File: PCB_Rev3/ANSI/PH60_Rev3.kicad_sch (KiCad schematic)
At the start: 50 parts, among them J1 USB_C_Receptacle_USB2.0_16P, J2 Conn_01x02, J3 Conn_01x02_Pin, J4 Conn_01x02_Pin, J6 Conn_01x02_Pin, J8 Conn_01x02_Pin, SW1 SW_SPDT_321, U1 TLV62569DBV, U2 RP2040, U4 ETA6093, U6 W25Q16JVSS, Y1 Crystal_GND24

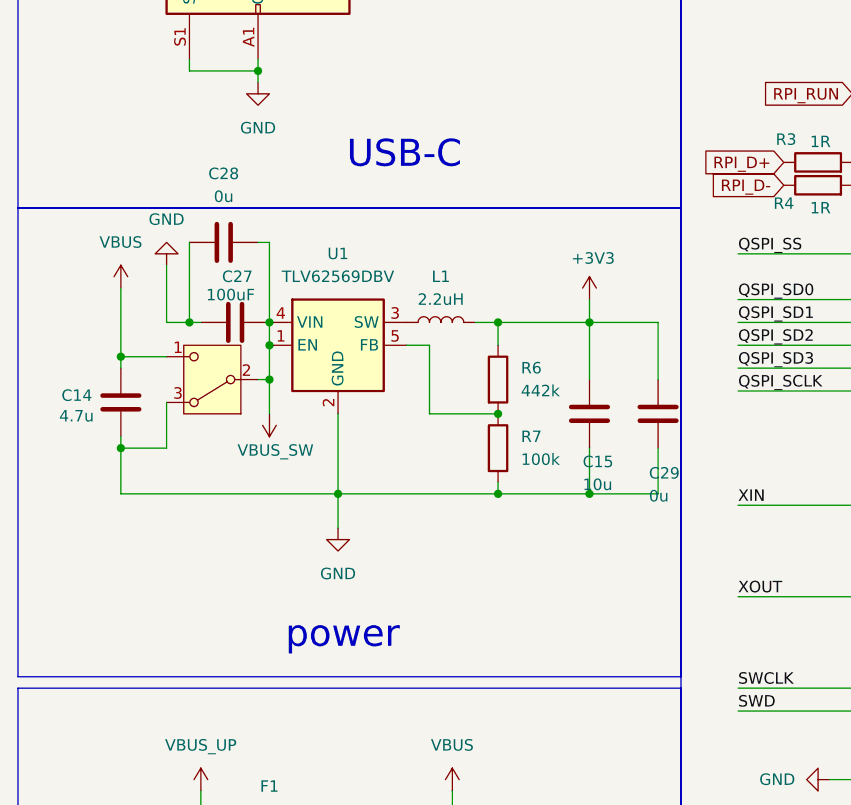
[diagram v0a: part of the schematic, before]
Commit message: Routing update
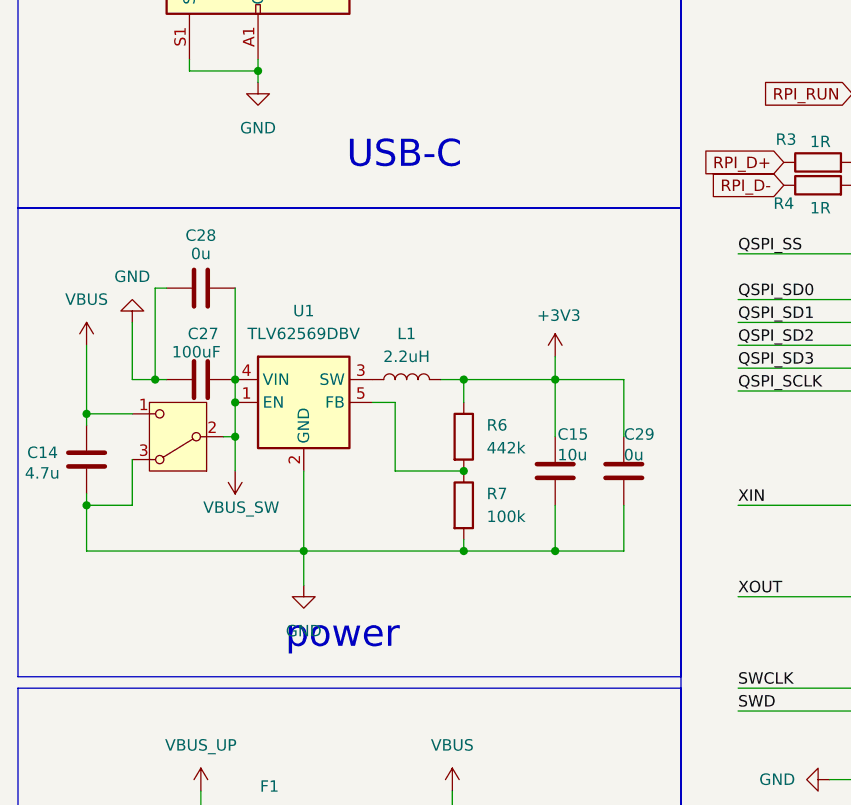
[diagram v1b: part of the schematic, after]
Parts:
- J4: footprint Connector_PinHeader_2.00mm:PinHeader_1x02_P2.00mm_Vertical -> Connector_PinHeader_1.27mm:PinHeader_1x02_P1.27mm_Vertical
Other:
- moved on the sheet: C14, C15, C27, C28, C29, L1, R6, R7, U1

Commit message: drc确认
1
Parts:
- C28, C29: now left out of the parts list
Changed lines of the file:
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@@
 		(unit 1)
 		(exclude_from_sim no)
-		(in_bom yes)
+		(in_bom no)
 		(on_board yes)
 		(dnp no)
@@
 		(unit 1)
 		(exclude_from_sim no)
-		(in_bom yes)
+		(in_bom no)
 		(on_board yes)
 		(dnp no)
